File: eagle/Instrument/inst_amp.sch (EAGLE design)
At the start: 12 parts, among them IC1 INA126U, X1 VCC +/-, X2 Vin, X3 Vout

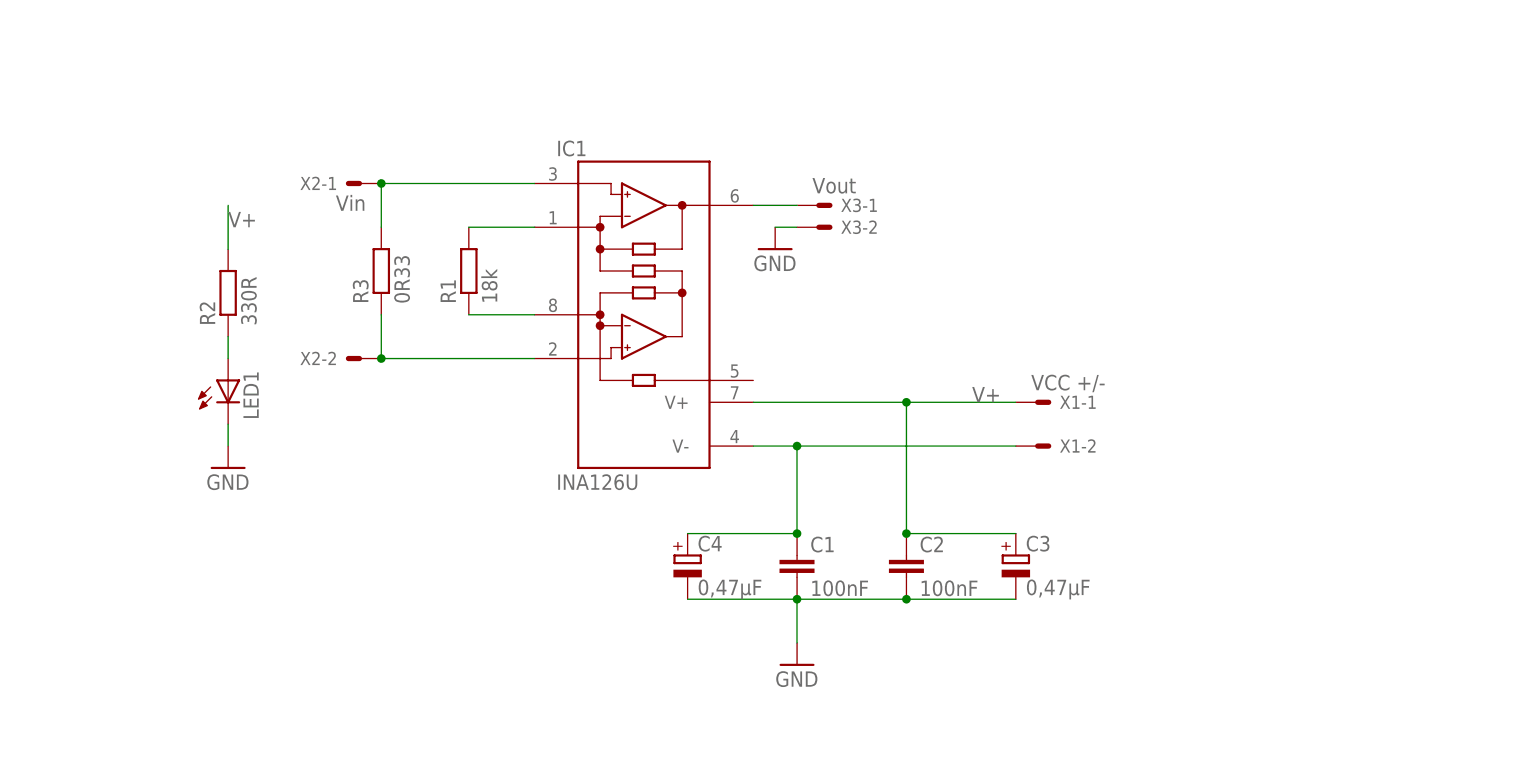
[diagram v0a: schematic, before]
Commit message: PCB design done
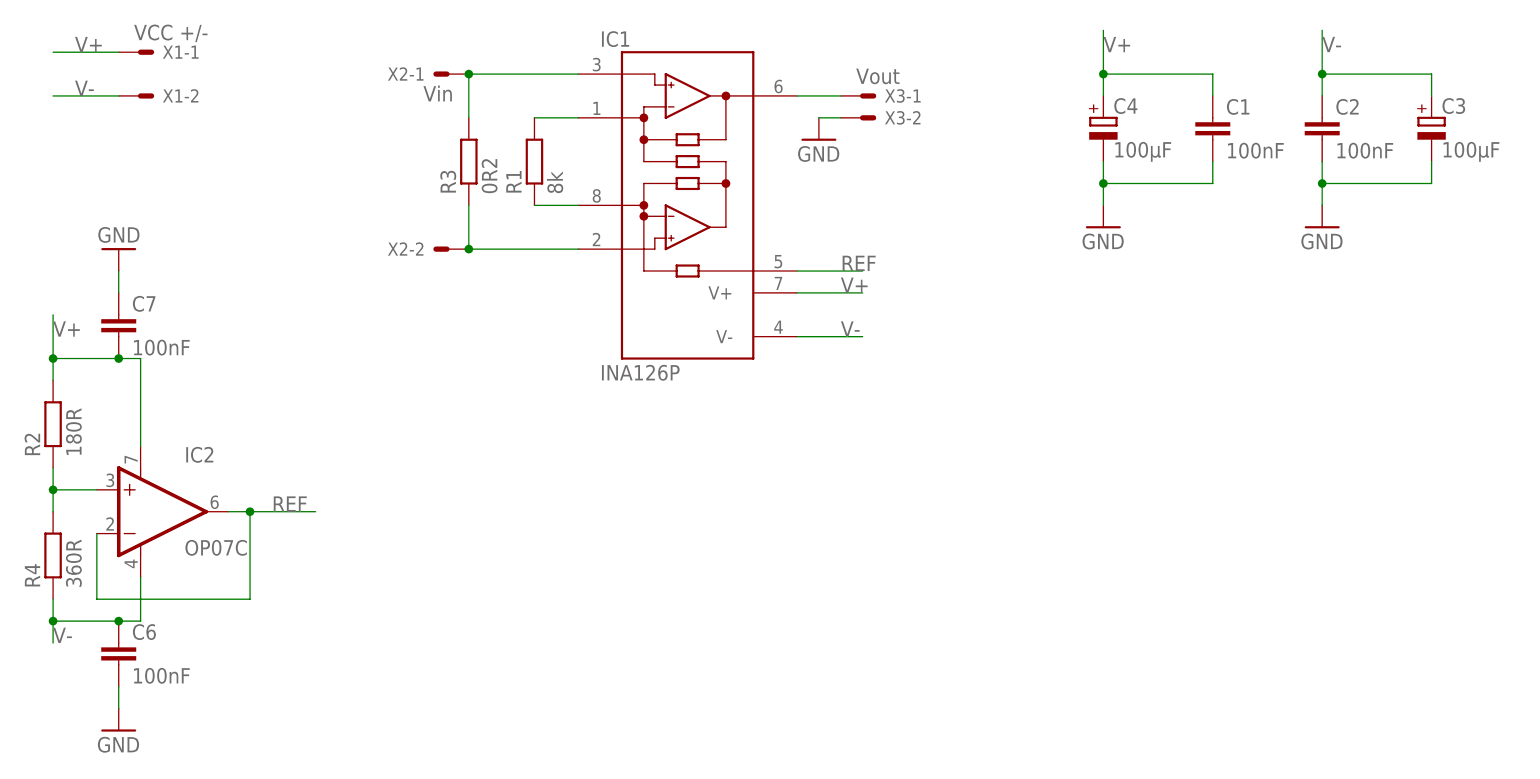
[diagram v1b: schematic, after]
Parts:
- removed LED1: (no value), led:LEDCHIPLED_1206
- added C6, C7: 100nF, rcl:C-EU050-025X075
- added IC2: OP07C, burr-brown:OPA658P
- added R4: 360R, rcl:R-EU_0207/10
- C1, C2: device rcl:C-EUC1206 -> rcl:C-EU050-025X075
- C3, C4: value 0,47µF -> 100µF; device rcl:CPOL-EU153CLV-0405 -> rcl:CPOL-EUE5-10.5
- IC1: value INA126U -> INA126P; device burr-brown:INA126U -> burr-brown:INA126P
- R1: value 18k -> 8k; device resistor:R-EU_R1206 -> rcl:R-EU_0207/10
- R2: value 330R -> 180R; device resistor:R-EU_R1206 -> rcl:R-EU_0207/10
- R3: value 0R33 -> 0R2; device rcl:R-EU_VTA55 -> rcl:R-EU_0414/15
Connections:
- removed net N$3: C1.1, C4.+, IC1.V-, X1-2.S
- removed net N$8: LED1.A, R2.1
- new net N$4: IC2.+IN, R2.1, R4.2
- new net REF: IC1.REF, IC2.-IN, IC2.OUT
- new net V-: C2.1, C3.+, C6.1, IC1.V-, IC2.V-, R4.1, X1-2.S
- net GND: now also C6.2, C7.1; no longer LED1.C
- net V+: now also C1.1, C4.+, C7.2, IC2.V+; no longer C2.1, C3.+
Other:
- moved on the sheet: C1, C2, C3, C4, IC1, R1, R2, R3, X1-1, X1-2, X2-1, X2-2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
